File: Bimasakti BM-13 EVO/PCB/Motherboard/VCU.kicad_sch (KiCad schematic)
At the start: 26 parts, among them J1 6437288-3, J10 power, J11 6437288-3, J2 12V, J3 3V3_1, J4 5V_5, J5 5V_1, J6 5V_2, J7 5V_3, J8 SIGNAL 1, J9 SIGNAL 2

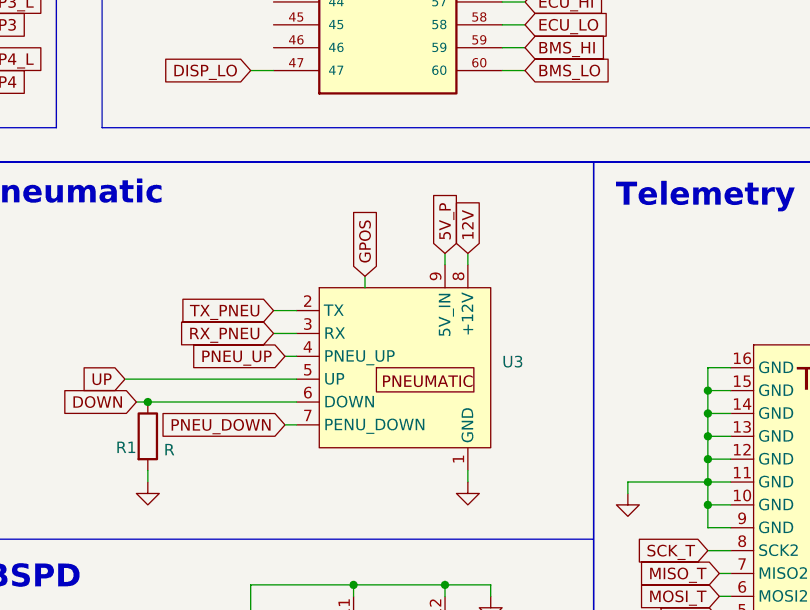
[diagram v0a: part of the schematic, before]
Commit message: update tv board
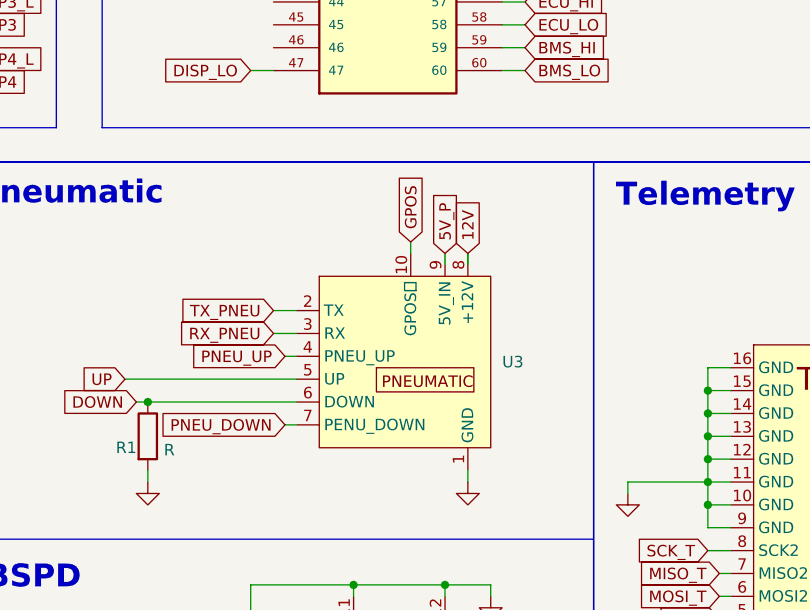
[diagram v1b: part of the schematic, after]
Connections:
- net GPOS: now also U3.10 (GPOS )
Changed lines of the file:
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@@
 	(wire
 		(pts
-			(xy 289.56 213.36) (xy 289.56 214.63)
-		)
-		(stroke
-			(width 0)
-			(type default)
-		)
-	)
-	(wire
-		(pts
 			(xy 181.61 173.99) (xy 179.07 173.99)
 		)
@@
 	(wire
 		(pts
+			(xy 294.64 209.55) (xy 294.64 210.82)
+		)
+		(stroke
+			(width 0)
+			(type default)
+		)
+	)
+	(wire
+		(pts
 			(xy 328.93 246.38) (xy 330.2 246.38)
 		)
@@
 	(global_label "GPOS"
 		(shape input)
-		(at 289.56 213.36 90)
+		(at 294.64 209.55 90)
 		(fields_autoplaced yes)
 		(effects
@@
 		)
 		(property "Intersheetrefs" "${INTERSHEET_REFS}"
-			(at 289.56 205.2948 90)
+			(at 294.64 201.4848 90)
 			(effects
 				(font
@@
 		(pin "3"
 		)
+		(pin "10"
+		)
 		(instances
